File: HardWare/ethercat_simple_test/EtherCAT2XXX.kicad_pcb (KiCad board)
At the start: 2 copper layers, 46.6 x 70.3 mm, 138 parts, among them CN1 5019530507, CN2 5019530507, J2 Conn_01x03, J3 Conn_01x04, J4 Conn_01x02, J5 Conn_01x02, J6 Conn_01x03, J7 Conn_01x04, J8 USB_C_Receptacle_USB2.0, SW1 SW_Push, U2 RT8075, U3 SRV05-4, U4 SRV05-4, U5 STM32F407VETx, U6 TJA1051T-3, U7 TJA1051T-3, U8 AX58100-LQPF80, U9 BL24C16F-PARC, X1 25M, Y1 8M, Y2 32.768KHz

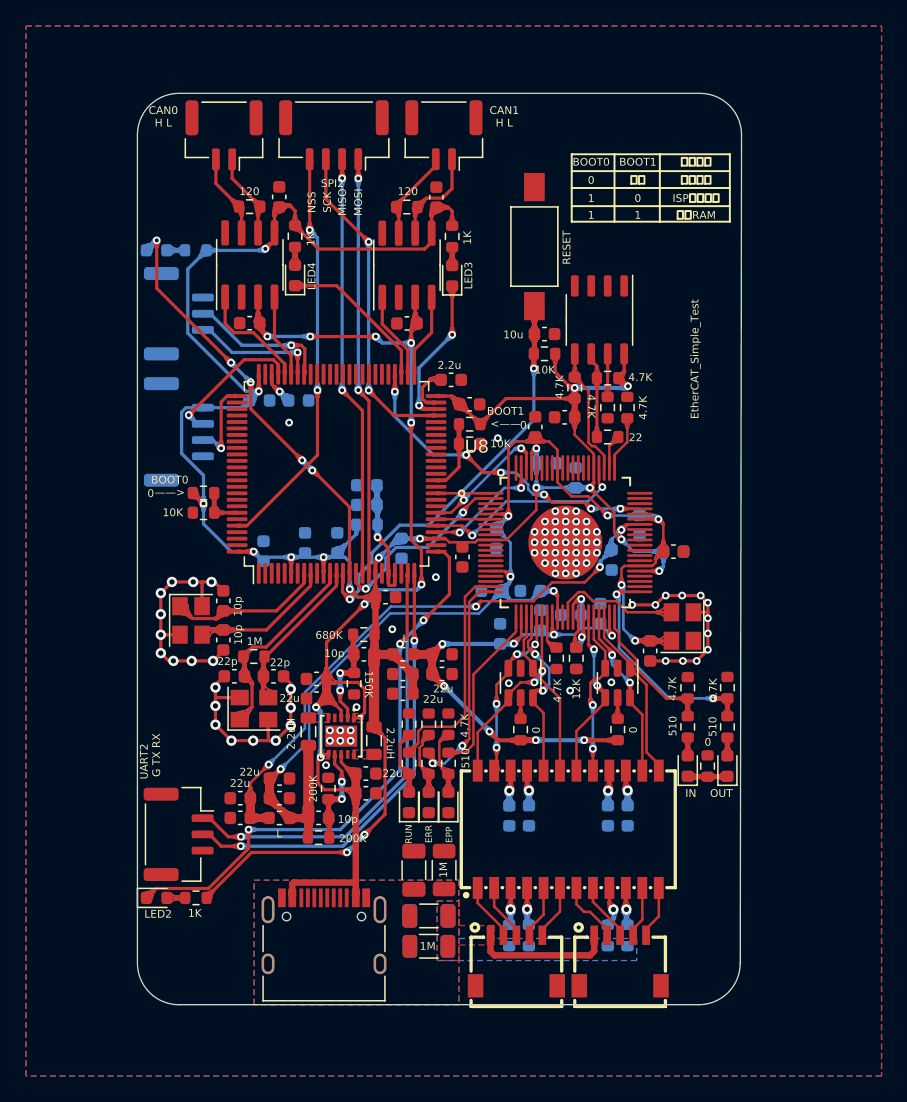
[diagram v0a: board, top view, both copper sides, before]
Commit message: Update gitignore
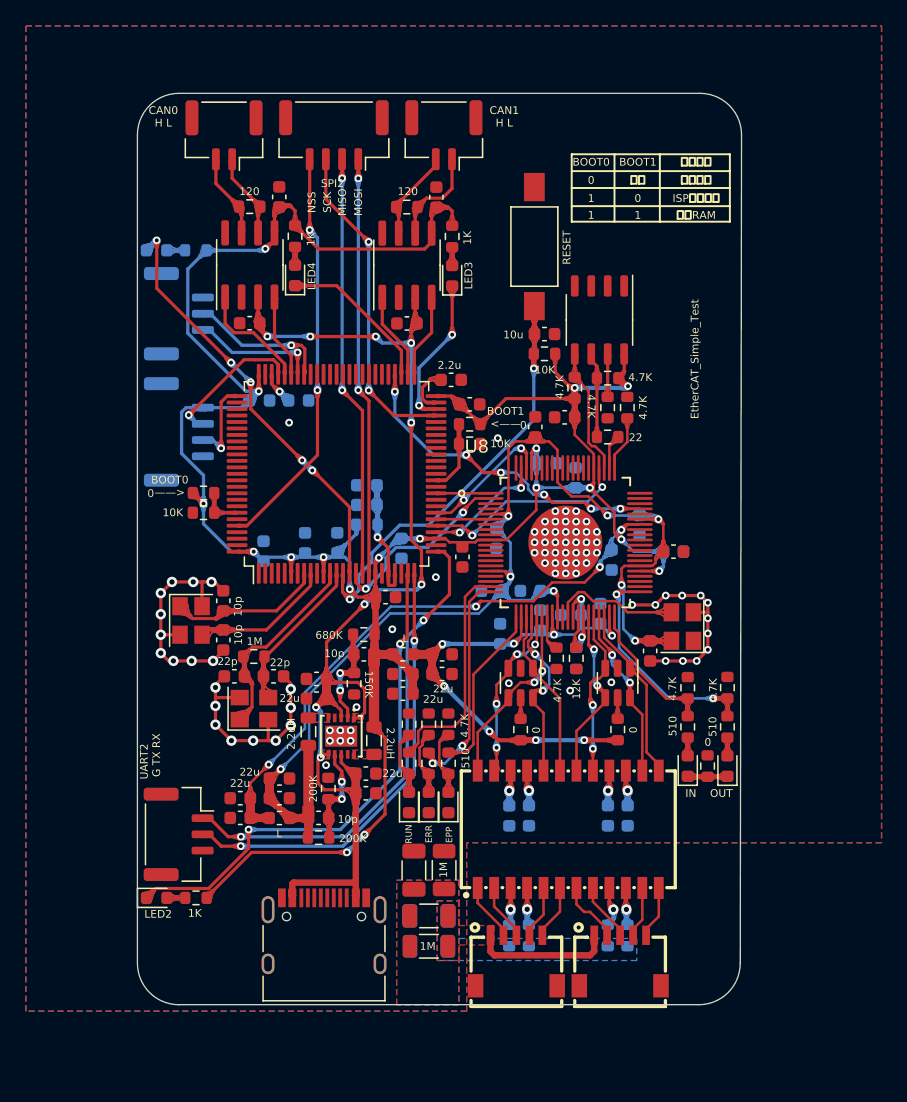
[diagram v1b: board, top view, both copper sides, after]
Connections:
- J8 pad A1: Earth -> GND
- J8 pad A12: Earth -> GND
- J8 pad B1: Earth -> GND
- J8 pad B12: Earth -> GND
- J8 pad S1: Earth -> GND
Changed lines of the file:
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@@
     (pad "" np_thru_hole circle (at 2.89 -2.6) (size 0.65 0.65) (drill 0.65) (layers "*.Cu" "*.Mask"))
     (pad "A1" smd rect (at -3.25 -4.045) (size 0.6 1.45) (layers "F.Cu" "F.Paste" "F.Mask")
-      (net 10 "Earth") (pinfunction "GND") (pintype "passive"))
+      (net 1 "GND") (pinfunction "GND") (pintype "passive"))
     (pad "A4" smd rect (at -2.45 -4.045) (size 0.6 1.45) (layers "F.Cu" "F.Paste" "F.Mask")
       (net 5 "+5V") (pinfunction "VBUS") (pintype "passive"))
@@
       (net 5 "+5V") (pinfunction "VBUS") (pintype "passive"))
     (pad "A12" smd rect (at 3.25 -4.045) (size 0.6 1.45) (layers "F.Cu" "F.Paste" "F.Mask")
-      (net 10 "Earth") (pinfunction "GND") (pintype "passive"))
+      (net 1 "GND") (pinfunction "GND") (pintype "passive"))
     (pad "B1" smd rect (at 3.25 -4.045) (size 0.6 1.45) (layers "F.Cu" "F.Paste" "F.Mask")
-      (net 10 "Earth") (pinfunction "GND") (pintype "passive"))
+      (net 1 "GND") (pinfunction "GND") (pintype "passive"))
     (pad "B4" smd rect (at 2.45 -4.045) (size 0.6 1.45) (layers "F.Cu" "F.Paste" "F.Mask")
       (net 5 "+5V") (pinfunction "VBUS") (pintype "passive"))
@@
       (net 5 "+5V") (pinfunction "VBUS") (pintype "passive"))
     (pad "B12" smd rect (at -3.25 -4.045) (size 0.6 1.45) (layers "F.Cu" "F.Paste" "F.Mask")
-      (net 10 "Earth") (pinfunction "GND") (pintype "passive"))
+      (net 1 "GND") (pinfunction "GND") (pintype "passive"))
     (pad "S1" thru_hole oval (at -4.32 -3.13) (size 1 2.1) (drill oval 0.6 1.7) (layers "*.Cu" "*.Mask")
-      (net 10 "Earth") (pinfunction "SHIELD") (pintype "passive"))
+      (net 1 "GND") (pinfunction "SHIELD") (pintype "passive"))
     (pad "S1" thru_hole oval (at -4.32 1.05) (size 1 1.6) (drill oval 0.6 1.2) (layers "*.Cu" "*.Mask")
-      (net 10 "Earth") (pinfunction "SHIELD") (pintype "passive"))
+      (net 1 "GND") (pinfunction "SHIELD") (pintype "passive"))
     (pad "S1" thru_hole oval (at 4.32 -3.13) (size 1 2.1) (drill oval 0.6 1.7) (layers "*.Cu" "*.Mask")
-      (net 10 "Earth") (pinfunction "SHIELD") (pintype "passive"))
+      (net 1 "GND") (pinfunction "SHIELD") (pintype "passive"))
     (pad "S1" thru_hole oval (at 4.32 1.05) (size 1 1.6) (drill oval 0.6 1.2) (layers "*.Cu" "*.Mask")
-      (net 10 "Earth") (pinfunction "SHIELD") (pintype "passive"))
+      (net 1 "GND") (pinfunction "SHIELD") (pintype "passive"))
     (model "${KICAD6_3DMODEL_DIR}/Connector_USB.3dshapes/USB_C_Receptacle_HRO_TYPE-C-31-M-12.wrl"
       (offset (xyz 0 0 0))
@@
     (polygon
       (pts
-        (xy 141 134)
-        (xy 75 134)
+        (xy 141 116)
+        (xy 109 116)
+        (xy 109 129)
+        (xy 75 129)
         (xy 75 53)
         (xy 141 53)
@@
       (pts
         (xy 108.4 128.5)
-        (xy 92.6 128.5)
-        (xy 92.6 118.9)
+        (xy 103.6 128.5)
+        (xy 103.6 118.9)
         (xy 108.4 118.9)
       )
